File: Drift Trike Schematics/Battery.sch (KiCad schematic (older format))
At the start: 121 parts

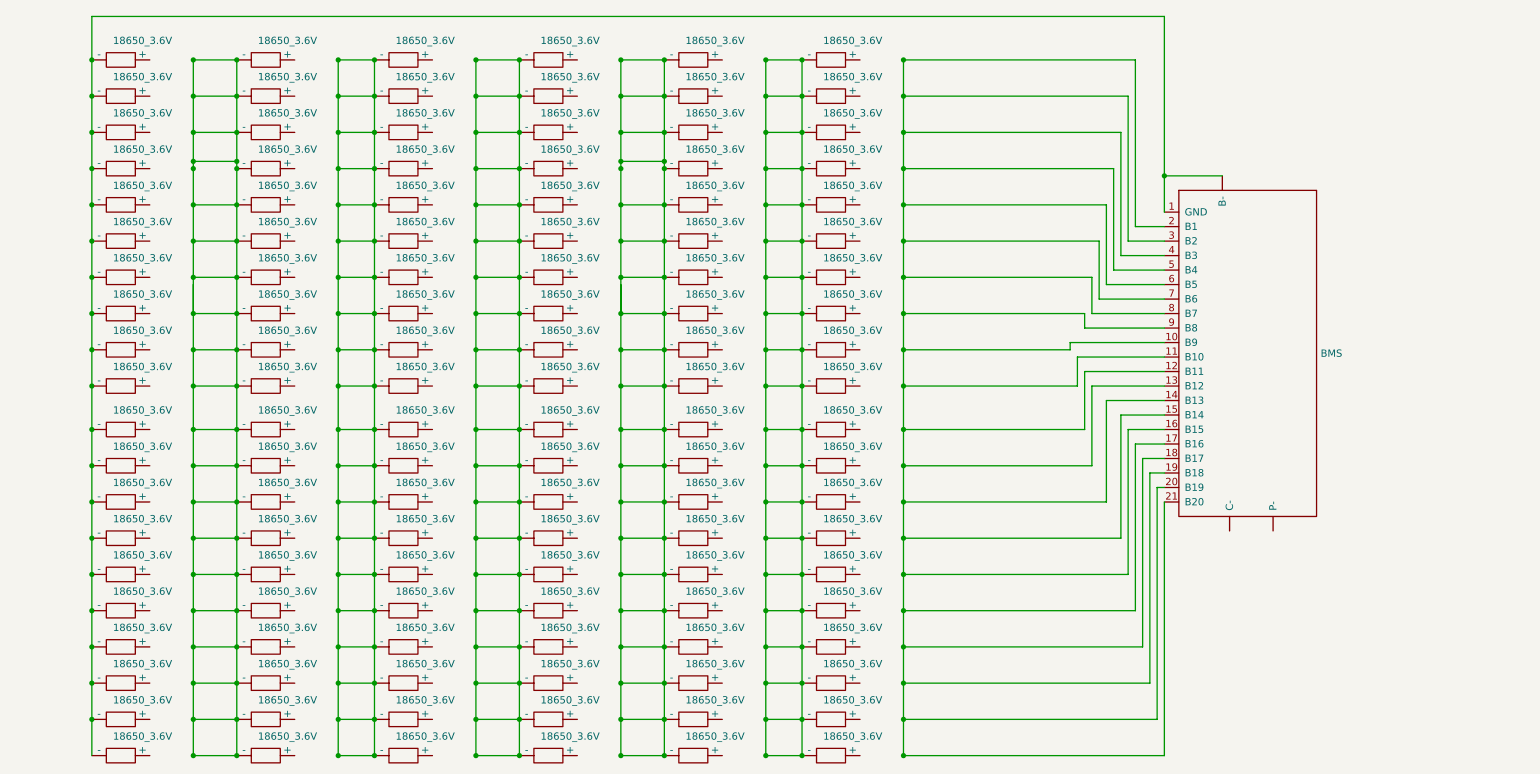
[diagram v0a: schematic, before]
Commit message: Battery
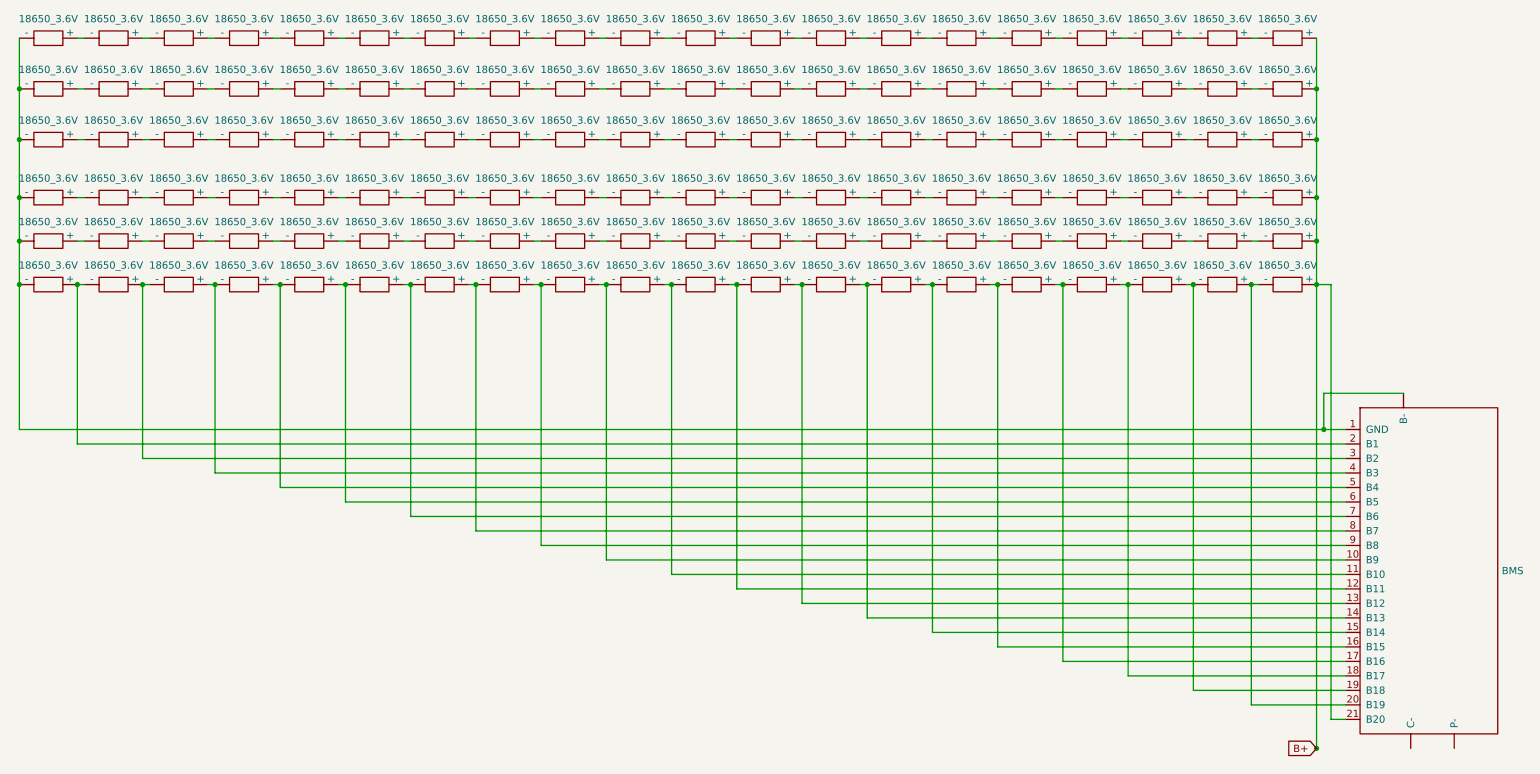
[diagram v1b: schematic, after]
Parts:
- removed U? (x120): 18650_3.6V, symbol trike_lib:18650_3.6V
- added U? (x120): 18650_3.6V, symbol trike_lib:18650_3.6V
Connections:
- net at U?.1 (GND), U?.~ (P-): now also U?.~ (-), U?.~ (-), U?.~ (-), U?.~ (-), U?.~ (-), U?.~ (-)
- new net: U?.10 (B9), U?.~ (-), U?.~ (-)
- new net: U?.11 (B10), U?.~ (-), U?.~ (-)
- new net: U?.12 (B11), U?.~ (-), U?.~ (-)
- new net: U?.13 (B12), U?.~ (-), U?.~ (-)
- new net: U?.14 (B13), U?.~ (-), U?.~ (-)
- new net: U?.15 (B14), U?.~ (-), U?.~ (-)
- new net: U?.16 (B15), U?.~ (-), U?.~ (-)
- new net: U?.17 (B16), U?.~ (-), U?.~ (-)
- new net: U?.18 (B17), U?.~ (-), U?.~ (-)
- new net: U?.19 (B18), U?.~ (-), U?.~ (-)
- new net: U?.2 (B1), U?.~ (-), U?.~ (-)
- new net: U?.20 (B19), U?.~ (-), U?.~ (-)
- new net: U?.3 (B2), U?.~ (-), U?.~ (-)
- new net: U?.4 (B3), U?.~ (-), U?.~ (-)
- new net: U?.5 (B4), U?.~ (-), U?.~ (-)
- new net: U?.6 (B5), U?.~ (-), U?.~ (-)
- new net: U?.7 (B6), U?.~ (-), U?.~ (-)
- new net: U?.8 (B7), U?.~ (-), U?.~ (-)
- new net: U?.9 (B8), U?.~ (-), U?.~ (-)
- new net: U?.~ (-), U?.~ (-) (x95)
- new net B+: U?.21 (B20), U?.~ (-), U?.~ (-), U?.~ (-), U?.~ (-), U?.~ (-), U?.~ (-)
